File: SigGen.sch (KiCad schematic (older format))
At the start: 19 parts, among them IC1 ATTINY2313-P, U1 4N25, U2 4N25, U3 DCDC_5V/5V

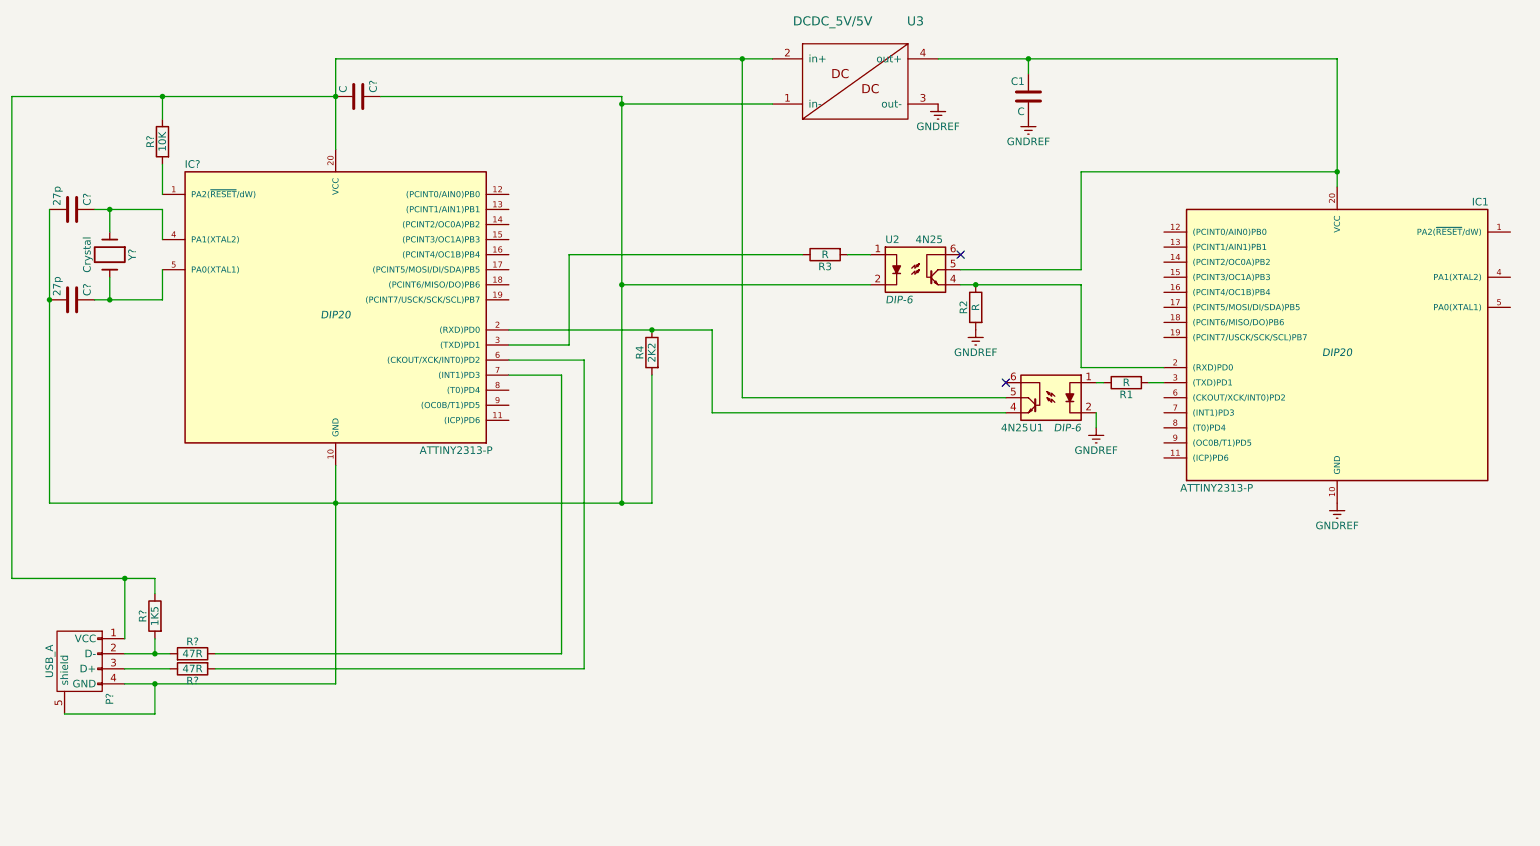
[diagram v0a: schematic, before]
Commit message: Updated schematic
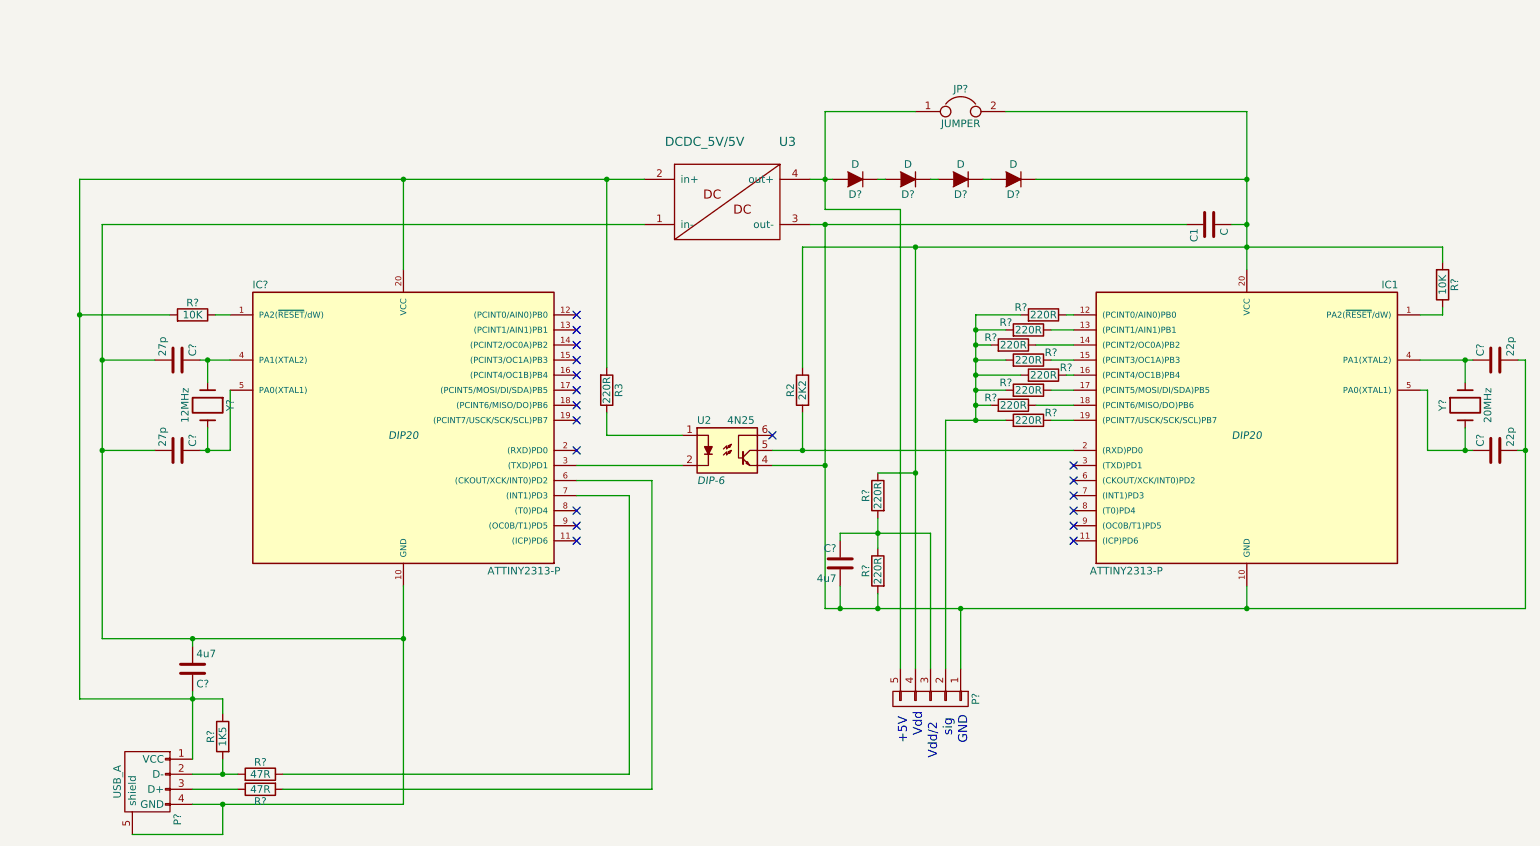
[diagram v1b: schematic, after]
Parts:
- removed R1: R, symbol R
- removed R4: 2K2, symbol R
- removed U1: 4N25, DIP-6, symbol 4N25
- added C?: 4u7, symbol C
- added C? (x2): 22p, symbol C
- added D? (x4): D, symbol D
- added JP?: JUMPER, symbol JUMPER
- added P?: CONN_01X05, symbol CONN_01X05
- added R?: 10K, symbol R
- added R? (x10): 220R, symbol R
- added Y?: 20MHz, symbol Crystal
- C?: value C -> 4u7
- R2: value R -> 2K2
- R3: value R -> 220R
- Y?: value Crystal -> 12MHz
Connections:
- net at IC1.1 (PA2(~RESET~/dW)): now also R?.1
- net at IC1.12 ((PCINT0/AIN0)PB0): now also R?.1
- net at IC1.13 ((PCINT1/AIN1)PB1): now also R?.1
- net at IC1.14 ((PCINT2/OC0A)PB2): now also R?.1
- net at IC1.15 ((PCINT3/OC1A)PB3): now also R?.1
- net at IC1.16 ((PCINT4/OC1B)PB4): now also R?.1
- net at IC1.17 ((PCINT5/MOSI/DI/SDA)PB5): now also R?.1
- net at IC1.18 ((PCINT6/MISO/DO)PB6): now also R?.1
- net at IC1.19 ((PCINT7/USCK/SCK/SCL)PB7): now also R?.1
- net at IC1.4 (PA1(XTAL2)): now also C?.1, Y?.1
- net at IC1.5 (PA0(XTAL1)): now also C?.1, Y?.2
- net at C?.2, C?.2, IC?.10 (GND)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: now also C?.2; no longer C?.1, U2.2
- net at IC?.20 (VCC), P?.1 (VCC), R?.1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: now also C?.1, R3.2, R?.2; no longer C?.2, R?.1
- net at U2.1: now also R3.1; no longer R3.2
- net at IC?.3 ((TXD)PD1): now also U2.2; no longer R3.1
- net at IC?.1 (PA2(~RESET~/dW)): now also R?.1; no longer R?.2
- net GNDREF: no longer names the net of IC1.10 (GND), U3.3 (out-)
- net GNDREF: now also C1.1, U2.4, C?.2, C?.2, C?.2, P?.1 (P1), R?.2; no longer C1.2, R2.2
- new net: IC1.2 ((RXD)PD0), R2.2, U2.5
- new net: C1.2, D?.1 (K), IC1.20 (VCC), JP?.2, P?.4 (P4), R2.1, R?.1, R?.2
- new net: D?.2 (A), JP?.1, P?.5 (P5), U3.4 (out+)
- new net: D?.1 (K), D?.2 (A) (x3)
- new net: P?.2 (P2), R?.2, R?.2, R?.2, R?.2, R?.2, R?.2, R?.2, R?.2
- new net: C?.1, P?.3 (P3), R?.1, R?.2
- no-connect marks 2 -> 19
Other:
- note added: "+5V"
- note added: "GND"
- note added: "Vdd"
- note added: "Vdd/2"
- note added: "sig"
- moved on the sheet: C1, C?, IC1, IC?, P?, R2, R3, R?, U2, U3, Y?
